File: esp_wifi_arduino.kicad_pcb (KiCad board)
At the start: 2 copper layers, 37 x 50 mm, 32 parts, among them IC1 ATMEGA328P-A, P1 CONN_15, P2 CONN_15, P3 CONN_1, P4 CONN_1, SW1 SW_PUSH, SW2 SW_PUSH, SW3 DIPSW4, U1 ADG3304, U2 ESP-WROOM-02, U3 NJM2391DL1-33, X1 16MHz

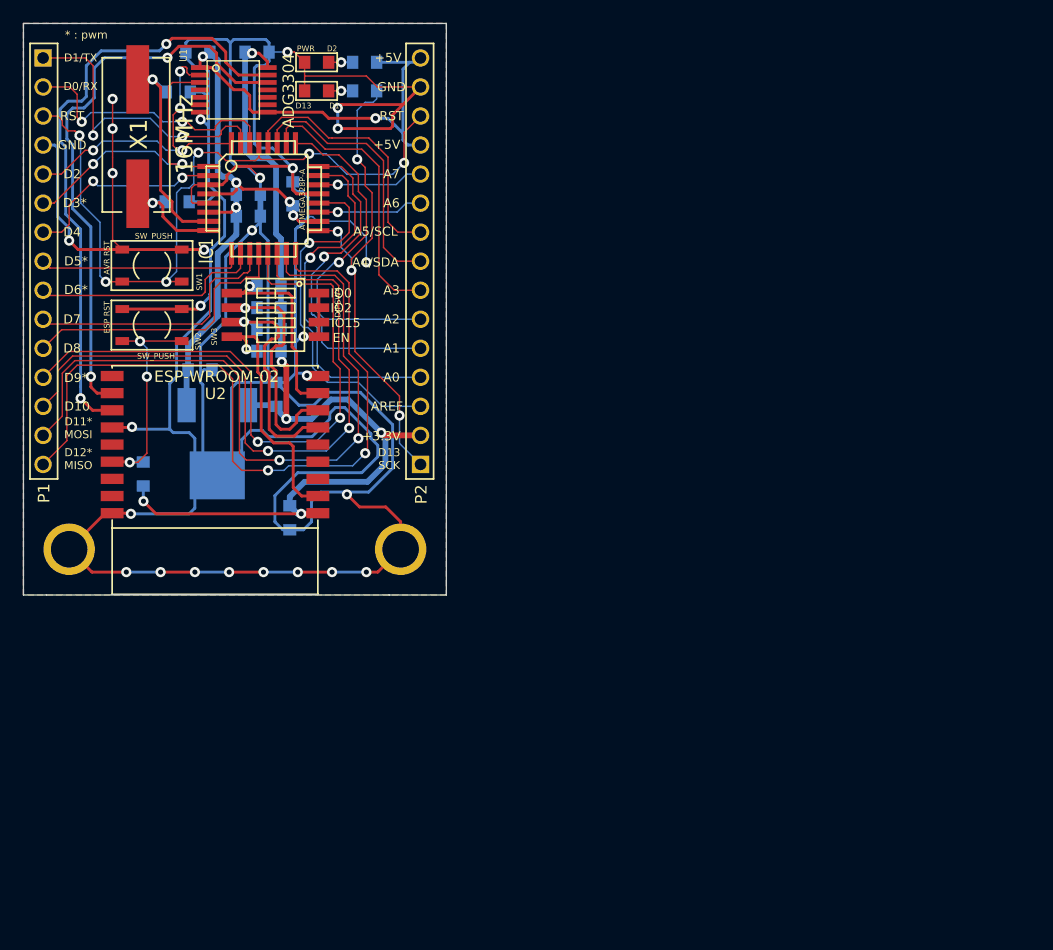
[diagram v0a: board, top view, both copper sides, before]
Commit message: PCB Layout
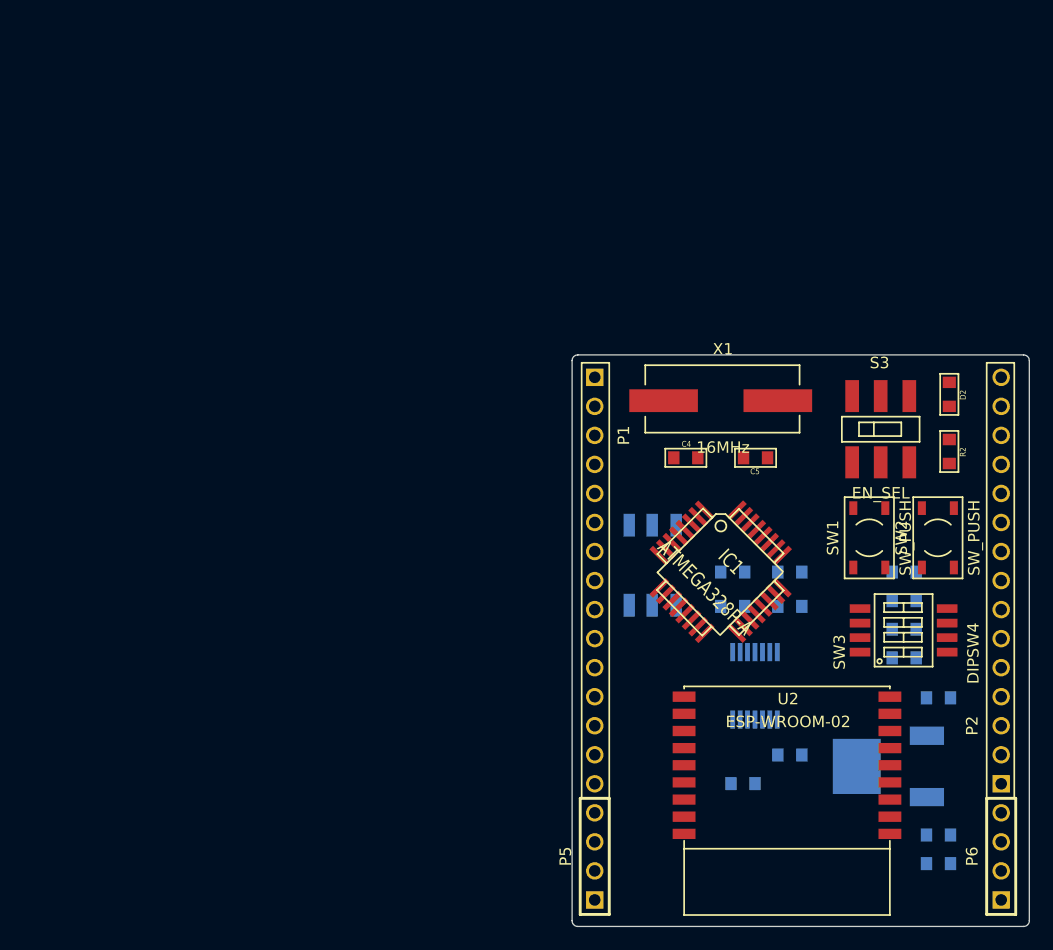
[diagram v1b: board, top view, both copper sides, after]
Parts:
- removed D1: LED, HANDSOL_0603
- removed G***: LOGO, LOGO
- removed P3, P4: CONN_1, M3_Drill
- removed R1: R, HANDSOL_0603
- added P5: CONN_01X04, PIN_ARRAY_4x1, F.Cu at (94.0, 102.9)
- added P6: CONN_01X04, PIN_ARRAY_4x1, F.Cu at (129.5, 102.9)
- added S1: RX_SEL, SEL, B.Cu at (99.0, 74.0)
- added S2: TX_SEL, SEL, B.Cu at (99.0, 81.0)
- added S3: EN_SEL, ALPS_SSSS213202(SlideSW), F.Cu at (119.0, 65.5)
- C4, C5, R2: moved to F.Cu
- P1, P2: value CONN_15 -> CONN_01X15
- U1: moved to B.Cu
- moved C7 77.2 mm to (111.0, 94.0)
- moved SW2 71.2 mm to (124.0, 75.0), turned to 90 degrees
- moved C6 70.9 mm to (111.0, 81.0), turned to 0 degrees
- moved C8 70.7 mm to (124.0, 89.0)
- moved C9 69.5 mm to (124.0, 101.0), turned to 0 degrees
- moved U1 69.3 mm to (108.0, 88.0), turned to 180 degrees
- moved SW1 67.1 mm to (118.0, 75.0), turned to 90 degrees
- moved C10 64.3 mm to (124.0, 103.5), turned to 0 degrees
- moved U3 64.3 mm to (119.0, 95.0), turned to 270 degrees
- moved SW3 63.3 mm to (121.0, 85.0), turned to 90 degrees
- moved D2 62.5 mm to (125.0, 62.5), turned to 90 degrees
- moved R5 62.5 mm to (121.0, 85.5), turned to 0 degrees
- moved R6 62.2 mm to (121.0, 83.0), turned to 0 degrees
- moved R7 61.9 mm to (121.0, 80.5), turned to 0 degrees
- moved R2 61.4 mm to (125.0, 67.5), turned to 90 degrees
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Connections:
- U1 pad 1: +5V -> +3.3V
- U1 pad 12: /ArduinoTX33 -> N-0000027
- U1 pad 13: /ArduinoRX33 -> N-0000026
- U1 pad 14: +3.3V -> +5V
- U1 pad 2: /D2 -> /ESP_TX
- U1 pad 3: /D3 -> /ESP_RX
- U1 pad 8: +5V -> N-0000011
- U2 pad 10: (no net) -> /IO4
- U2 pad 11: /ArduinoTX33 -> /ESP_RX
- U2 pad 12: /ArduinoRX33 -> /ESP_TX
- U2 pad 14: (no net) -> /IO5
- U2 pad 17: (no net) -> /IO16
- U2 pad 3: (no net) -> /IO14
- U2 pad 4: (no net) -> /IO12
- U2 pad 5: (no net) -> /IO13
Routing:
- net GND: track 401.0 -> 0.00 mm, vias 27 -> 0
- net +3.3V: track 86.4 -> 0.00 mm, vias 6 -> 0
- net +5V: track 84.4 -> 0.00 mm, vias 6 -> 0
- net /D12: track 65.9 -> 0.00 mm, vias 2 -> 0
- net /RESET: track 63.2 -> 0.00 mm, vias 6 -> 0
- net /D11: track 61.9 -> 0.00 mm, vias 2 -> 0
- net /D10: track 58.0 -> 0.00 mm, vias 2 -> 0
- net /D9: track 54.3 -> 0.00 mm, vias 2 -> 0
- net /ArduinoRX33: track 53.4 -> 0.00 mm, vias 2 -> 0
- net /ArduinoTX33: track 50.2 -> 0.00 mm, vias 2 -> 0
- net /D13: track 43.2 -> 0.00 mm, vias 4 -> 0
- net /A0: track 32.3 -> 0.00 mm, vias 1 -> 0
- net /AREF: track 31.7 -> 0.00 mm, vias 1 -> 0
- net /A2: track 30.3 -> 0.00 mm, vias 1 -> 0
- net /A1: track 29.9 -> 0.00 mm, vias 1 -> 0
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- removed copper zone on B.Cu, net GND
- removed copper zone on F.Cu, net GND
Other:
- board size 37 x 50 mm -> 40 x 50 mm
- rule trace_min: 0.127 -> 0.254
- board text removed: "* : pwm"
- board text removed: "+3.3V"
- board text removed: "+5V"
- board text removed: "A0"
- board text removed: "A1"
- board text removed: "A2"
- board text removed: "A3"
- board text removed: "A4/SDA"
- board text removed: "A5/SCL"
- board text removed: "A6"
- board text removed: "A7"
- board text removed: "AREF"
- board text removed: "AVR RST"
- board text removed: "Asumonoduino-Wifi"
- board text removed: "D0/RX"
- board text removed: "D1/TX"
- board text removed: "D10"
- board text removed: "D11* MOSI"
- board text removed: "D12* MISO"
- board text removed: "D13"
- board text removed: "D13 SCK"
- board text removed: "D2"
- board text removed: "D2(SS RX)"
- board text removed: "D3(SS TX)"
- board text removed: "D3*"
- board text removed: "D4"
- board text removed: "D5*"
- board text removed: "D6*"
- board text removed: "D7"
- board text removed: "D8"
- board text removed: "D9*"
- board text removed: "EN"
- board text removed: "ESP RST"
- board text removed: "GND"
- board text removed: "IO0"
- board text removed: "IO15"
- board text removed: "IO2"
- board text removed: "PWR"
- board text removed: "RST"
